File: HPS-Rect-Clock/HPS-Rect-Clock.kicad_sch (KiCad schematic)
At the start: 48 parts, among them J1 Conn_01x06, J2 PJ-102AH, SW1 Omron_B3F_SPST, SW2 Omron_B3F_SPST, SW3 Omron_B3F_SPST, SW4 Omron_B3F_SPST, SW5 Omron_B3F_SPST, U1 DS1307_DIP-8, U2 ATmega328-PU, U3 L7805, Y1 Crystal_16MHz, Y2 Crystal_32768Hz

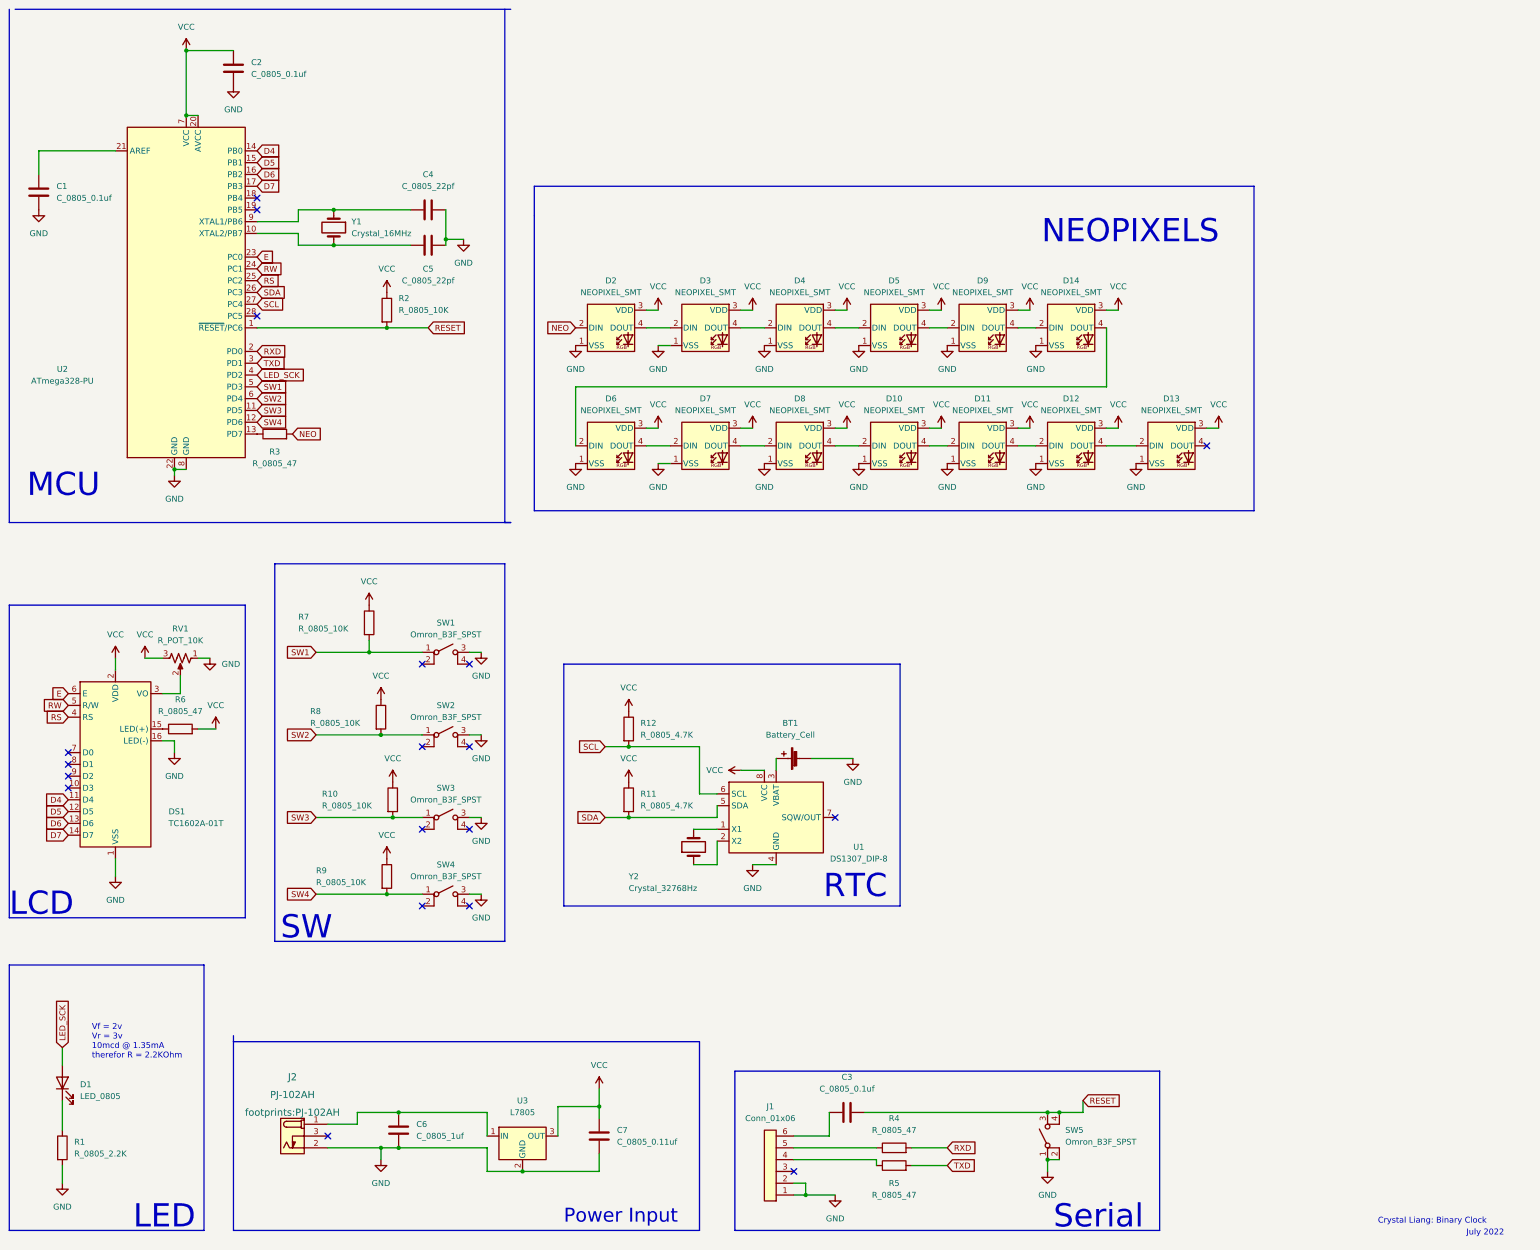
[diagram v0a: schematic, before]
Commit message: Week 6: Pre route
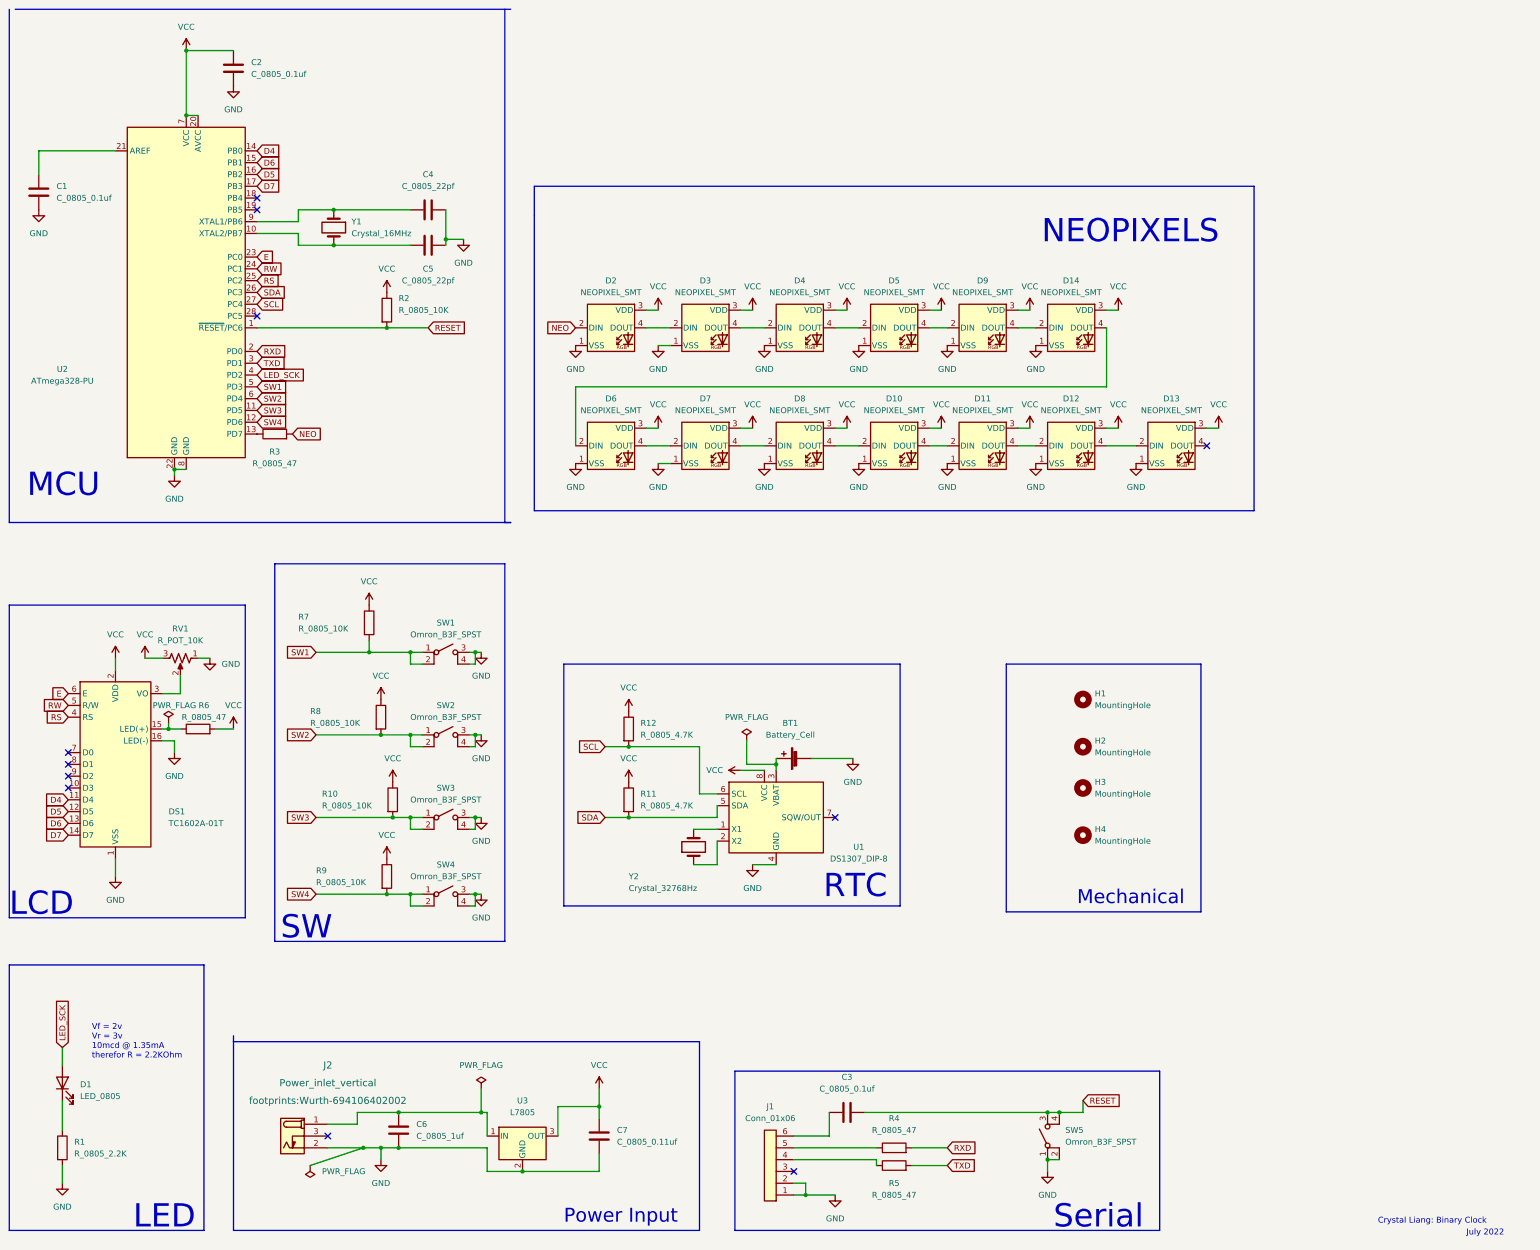
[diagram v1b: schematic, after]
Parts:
- removed J2: PJ-102AH, footprints:PJ-102AH, symbol HPS:PJ-102AH
- added H1, H2, H3, H4: MountingHole, footprints:MountingHole_3.2mm_M3, symbol HPS:MountingHole
- added J2: Power_inlet_vertical, footprints:Wurth-694106402002, symbol HPS:Power_inlet_vertical
- U3: footprint (none) -> footprints:TO-252-2; Digikey PN (none) -> 497-7255-1-ND; MFG (none) -> STMicroelectronics; MPN (none) -> L7805CDT-TR
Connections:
- net D5: now also U2.16 (PB2); no longer U2.15 (PB1)
- net D6: now also U2.15 (PB1); no longer U2.16 (PB2)
- net GND: now also SW1.4 (B), SW2.4 (B), SW3.4 (B), SW4.4 (B), J2.2 (OUT)
- net SW1: now also SW1.2 (A)
- net SW2: now also SW2.2 (A)
- net SW3: now also SW3.2 (A)
- net SW4: now also SW4.2 (A)
- net at C6.2, U3.1 (IN): now also J2.1 (POLE)
- no-connect marks 19 -> 11
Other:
- note added: "Mechanical"
- moved on the sheet: R6

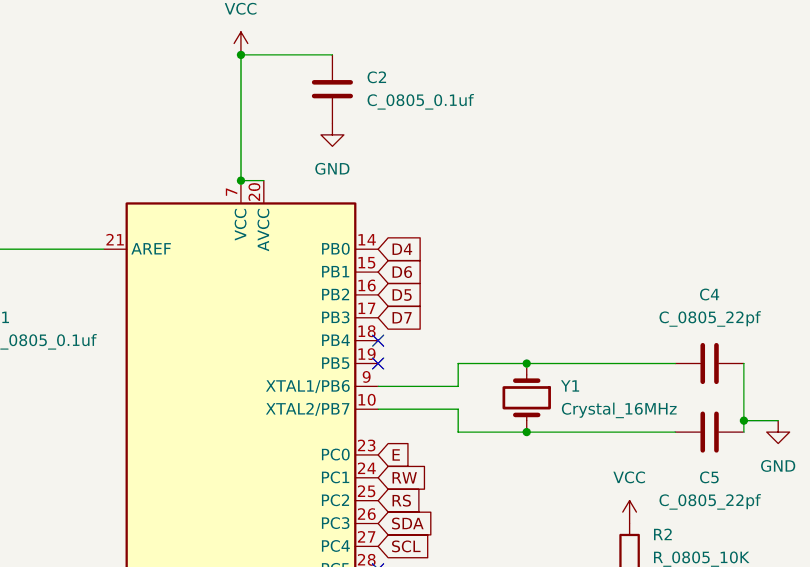
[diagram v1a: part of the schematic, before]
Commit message: PCB Placement Done
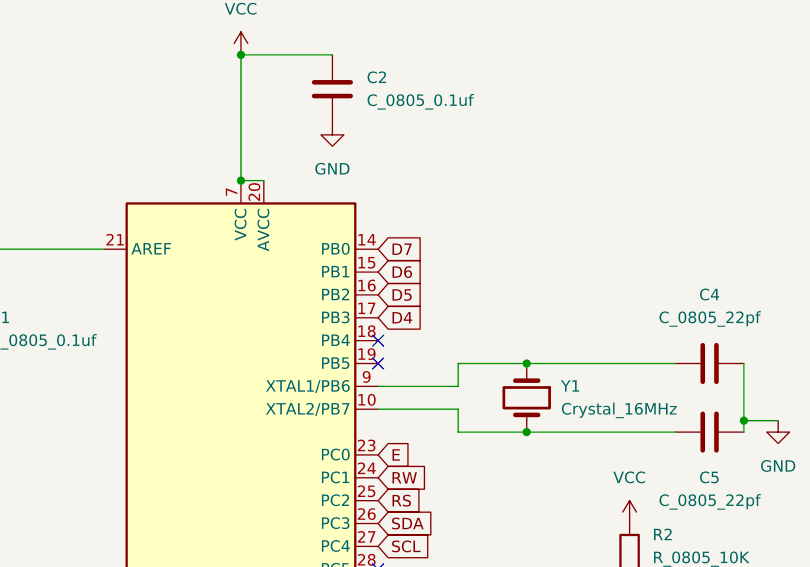
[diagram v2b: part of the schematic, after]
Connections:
- net D4: now also U2.17 (PB3); no longer U2.14 (PB0)
- net D7: now also U2.14 (PB0); no longer U2.17 (PB3)
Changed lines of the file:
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@@
     )
   )
-  (global_label "D4" (shape input) (at 69.85 46.99 0) (fields_autoplaced)
+  (global_label "D4" (shape input) (at 69.85 54.61 0) (fields_autoplaced)
     (effects (font (size 1.27 1.27)) (justify left))
-    (property "Intersheet References" "${INTERSHEET_REFS}" (id 0) (at 74.7426 47.0694 0)
+    (property "Intersheet References" "${INTERSHEET_REFS}" (id 0) (at 74.7426 54.6894 0)
       (effects (font (size 1.27 1.27)) (justify left) hide)
     )
@@
     )
   )
-  (global_label "D7" (shape input) (at 69.85 54.61 0) (fields_autoplaced)
+  (global_label "D7" (shape input) (at 69.85 46.99 0) (fields_autoplaced)
     (effects (font (size 1.27 1.27)) (justify left))
-    (property "Intersheet References" "${INTERSHEET_REFS}" (id 0) (at 74.7426 54.5306 0)
+    (property "Intersheet References" "${INTERSHEET_REFS}" (id 0) (at 74.7426 46.9106 0)
       (effects (font (size 1.27 1.27)) (justify left) hide)
     )

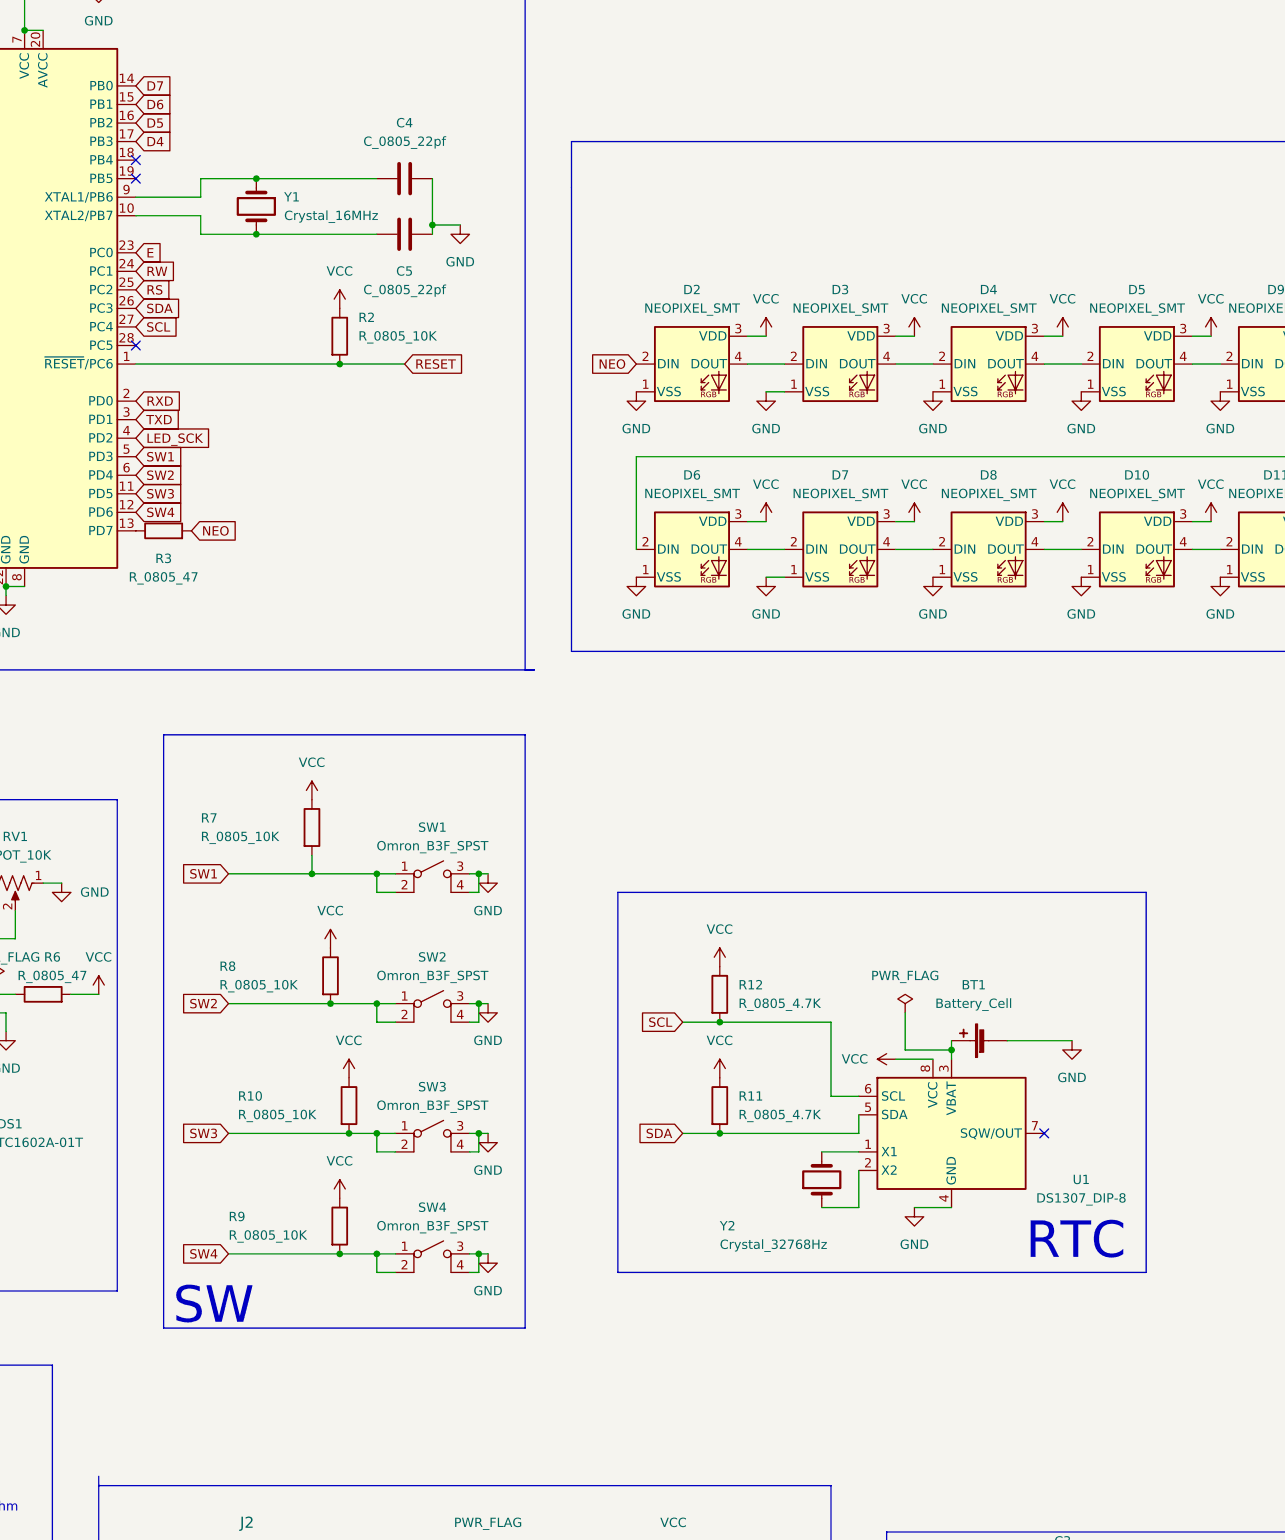
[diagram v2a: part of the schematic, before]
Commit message: Pre Gerber Edits
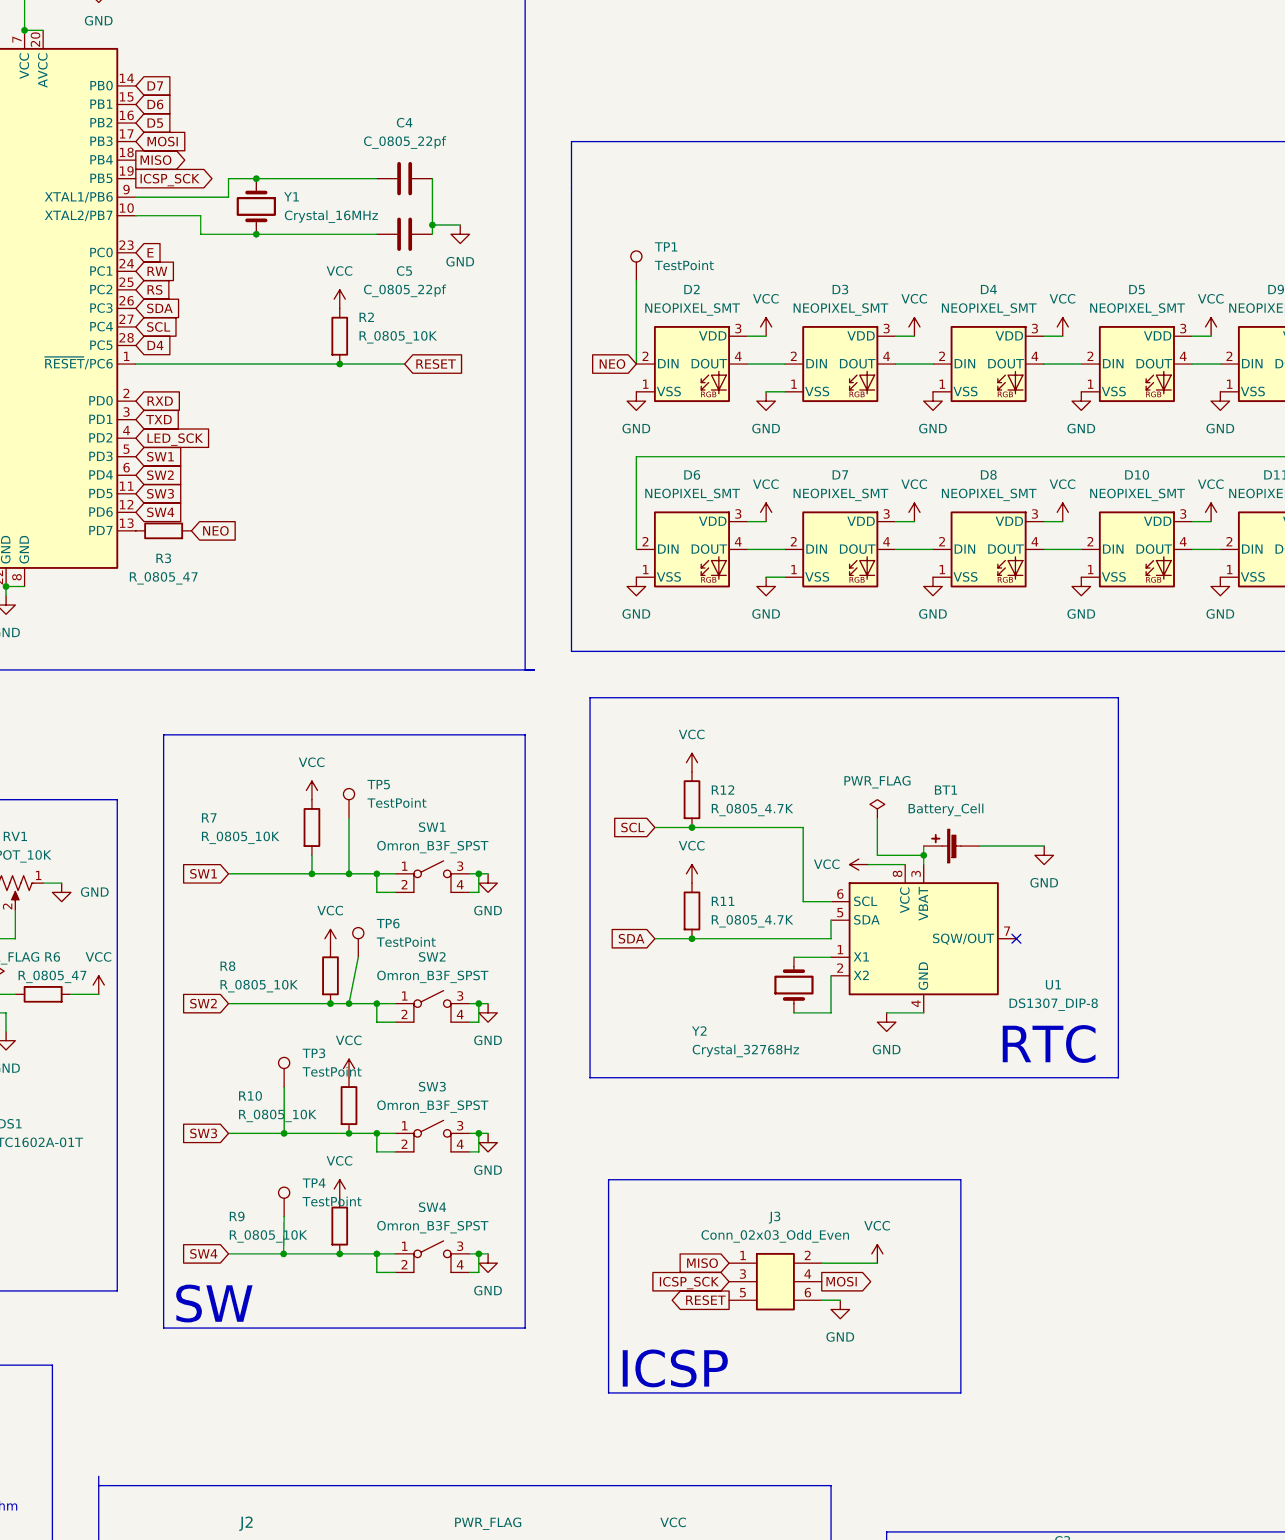
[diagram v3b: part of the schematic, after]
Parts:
- added J3: Conn_02x03_Odd_Even, footprints:PinHeader_2x03_P2.54mm_Vertical, symbol HPS:Conn_02x03_Odd_Even
- added TP1, TP3, TP4, TP5, TP6: TestPoint, footprints:TestPoint_THTPad_D2.0mm_Drill1.0mm, symbol HPS:TestPoint
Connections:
- net D4: now also U2.28 (PC5); no longer U2.17 (PB3)
- net GND: now also J3.6 (Pin_6)
- net NEO: now also TP1.1
- net RESET: now also J3.5 (Pin_5)
- net SW1: now also TP5.1
- net SW2: now also TP6.1
- net SW3: now also TP3.1
- net SW4: now also TP4.1
- net VCC: now also J3.2 (Pin_2)
- net MISO: now reaches U2.18 (PB4)
- net MISO: now also J3.1 (Pin_1)
- net ICSP_SCK: now reaches U2.19 (PB5)
- net ICSP_SCK: now also J3.3 (Pin_3)
- new net MOSI: J3.4 (Pin_4), U2.17 (PB3)
- no-connect marks 11 -> 8
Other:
- note added: "ICSP"
- moved on the sheet: BT1, R11, R12, U1, Y2
